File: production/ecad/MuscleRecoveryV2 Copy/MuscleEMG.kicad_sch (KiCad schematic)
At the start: 34 parts, among them J6 Screw_Terminal_01x03, U5 AD8232ACPZ-R7, U7 ADS1115IDGS

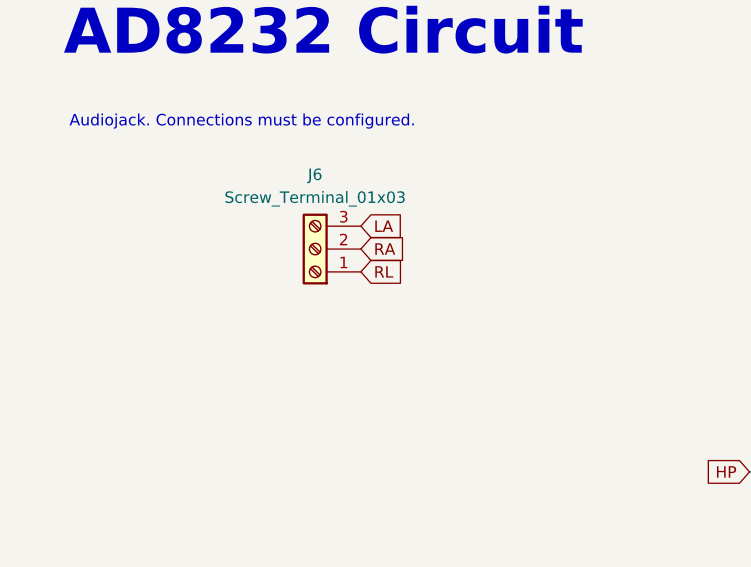
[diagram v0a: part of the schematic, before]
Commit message: Pushing Most of the final changes for PCB REV2
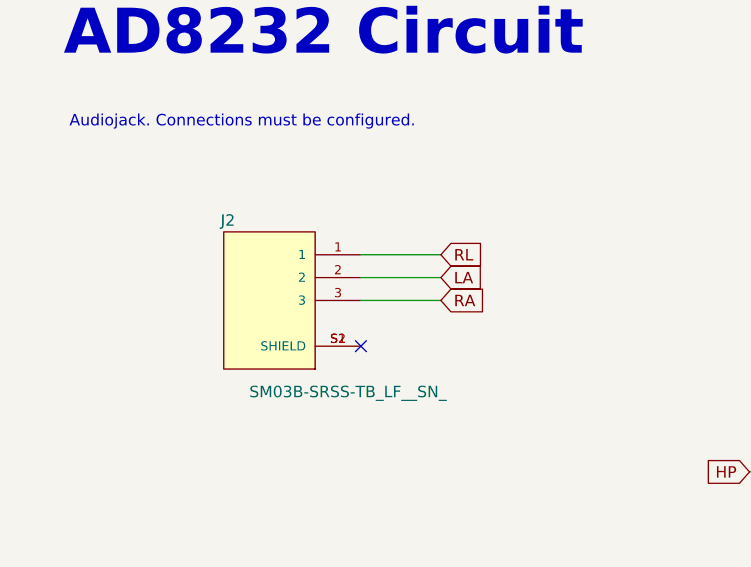
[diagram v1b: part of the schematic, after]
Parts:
- removed J6: Screw_Terminal_01x03, Connector_PinHeader_2.54mm:PinHeader_1x03_P2.54mm_Horizontal, symbol Connector:Screw_Terminal_01x03
- added J2: SM03B-SRSS-TB_LF__SN_, Muscle_Recovery_Footprint_Library:JST_SM03B-SRSS-TB_LF__SN_, symbol MuscleRecoverySymbolLibray:SM03B-SRSS-TB_LF__SN_
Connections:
- net LA: now also J2.2
- net RA: now also J2.3
- net RL: now also J2.1
- new net: J2.S1 (SHIELD), J2.S2 (SHIELD)
- no-connect marks 3 -> 4
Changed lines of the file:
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@@
   (no_connect (at 35.56 172.72))
   (no_connect (at 35.56 170.18))
+  (no_connect (at 52.07 60.96))
   (wire (pts (xy 119.38 52.07) (xy 119.38 49.53))
     (stroke (width 0) (type default))
@@
     (stroke (width 0) (type default))
   )
+  (wire (pts (xy 52.07 55.88) (xy 60.96 55.88))
+    (stroke (width 0) (type default))
+  )
   (wire (pts (xy 219.71 52.07) (xy 245.11 52.07))
     (stroke (width 0) (type default))
@@
     (stroke (width 0) (type default))
   )
+  (wire (pts (xy 52.07 53.34) (xy 60.96 53.34))
+    (stroke (width 0) (type default))
+  )
   (wire (pts (xy 119.38 35.56) (xy 124.46 35.56))
     (stroke (width 0) (type default))
@@
   )
   (wire (pts (xy 125.73 22.86) (xy 128.27 22.86))
+    (stroke (width 0) (type default))
+  )
+  (wire (pts (xy 52.07 50.8) (xy 60.96 50.8))
     (stroke (width 0) (type default))
   )
@@
   (text "ADC" (at 25.4 139.7 0)
     (effects (font (size 5 5) bold) (justify left bottom))
-  )
-  (global_label "RA" (shape input) (at 52.07 50.165 0) (fields_autoplaced)
-    (effects (font (size 1.27 1.27)) (justify left))
-    (property "Intersheetrefs" "${INTERSHEET_REFS}" (at 57.4138 50.165 0)
-      (effects (font (size 1.27 1.27)) (justify left) hide)
-    )
   )
   (global_label "SCL" (shape input) (at 76.2 170.18 0) (fields_autoplaced)
@@
     )
   )
+  (global_label "LA" (shape input) (at 60.96 53.34 0) (fields_autoplaced)
+    (effects (font (size 1.27 1.27)) (justify left))
+    (property "Intersheetrefs" "${INTERSHEET_REFS}" (at 66.0619 53.34 0)
+      (effects (font (size 1.27 1.27)) (justify left) hide)
+    )
+  )
   (global_label "SW" (shape input) (at 144.78 66.04 180) (fields_autoplaced)
     (effects (font (size 1.27 1.27)) (justify right))
@@
     )
   )
-  (global_label "RL" (shape input) (at 52.07 52.705 0) (fields_autoplaced)
-    (effects (font (size 1.27 1.27)) (justify left))
-    (property "Intersheetrefs" "${INTERSHEET_REFS}" (at 57.3533 52.705 0)
-      (effects (font (size 1.27 1.27)) (justify left) hide)
-    )
-  )
   (global_label "ALERT{slash}READY" (shape bidirectional) (at 226.06 156.21 180) (fields_autoplaced)
     (effects (font (size 1.27 1.27)) (justify right))
@@
     )
   )
-  (global_label "LA" (shape input) (at 52.07 47.625 0) (fields_autoplaced)
+  (global_label "RA" (shape input) (at 60.96 55.88 0) (fields_autoplaced)
     (effects (font (size 1.27 1.27)) (justify left))
-    (property "Intersheetrefs" "${INTERSHEET_REFS}" (at 57.1719 47.625 0)
+    (property "Intersheetrefs" "${INTERSHEET_REFS}" (at 66.3038 55.88 0)
       (effects (font (size 1.27 1.27)) (justify left) hide)
     )
@@
     )
   )
+  (global_label "RL" (shape input) (at 60.96 50.8 0) (fields_autoplaced)
+    (effects (font (size 1.27 1.27)) (justify left))
+    (property "Intersheetrefs" "${INTERSHEET_REFS}" (at 66.2433 50.8 0)
+      (effects (font (size 1.27 1.27)) (justify left) hide)
+    )
+  )
   (global_label "LOD+" (shape input) (at 219.71 71.12 0) (fields_autoplaced)
     (effects (font (size 1.27 1.27)) (justify left))
@@
         (path "/4e550305-79d2-4e4a-a502-817ebcc79f9a/284c60dd-e199-4b03-b99f-cc7eaed256f8"
           (reference "C3") (unit 1)
-        )
-      )
-    )
-  )
-  (symbol (lib_id "Connector:Screw_Terminal_01x03") (at 46.99 50.165 180) (unit 1)
-    (in_bom yes) (on_board yes) (dnp no) (fields_autoplaced)
-    (property "Reference" "J6" (at 46.99 41.91 0)
-      (effects (font (size 1.27 1.27)))
-    )
-    (property "Value" "Screw_Terminal_01x03" (at 46.99 44.45 0)
-      (effects (font (size 1.27 1.27)))
-    )
-    (property "Footprint" "Connector_PinHeader_2.54mm:PinHeader_1x03_P2.54mm_Horizontal" (at 46.99 50.165 0)
-      (effects (font (size 1.27 1.27)) hide)
-    )
-    (property "Datasheet" "~" (at 46.99 50.165 0)
-      (effects (font (size 1.27 1.27)) hide)
-    )
-    (pin "1")
-    (pin "2")
-    (pin "3")
-    (instances
-      (project "MuscleRecoveryV1"
-        (path "/4e550305-79d2-4e4a-a502-817ebcc79f9a/284c60dd-e199-4b03-b99f-cc7eaed256f8"
-          (reference "J6") (unit 1)
         )
       )
@@
         )
       )
+    )
+  )
+  (symbol (lib_id "MuscleRecoverySymbolLibray:SM03B-SRSS-TB_LF__SN_") (at 41.91 55.88 0) (mirror y) (unit 1)
+    (in_bom yes) (on_board yes) (dnp no)
+    (property "Reference" "J2" (at 38.1 46.99 0)
+      (effects (font (size 1.27 1.27)) (justify left))
+    )
+    (property "Value" "SM03B-SRSS-TB_LF__SN_" (at 61.595 66.04 0)
+      (effects (font (size 1.27 1.27)) (justify left))
+    )
+    (property "Footprint" "Muscle_Recovery_Footprint_Library:JST_SM03B-SRSS-TB_LF__SN_" (at 34.29 71.12 0)
+      (effects (font (size 1.27 1.27)) (justify bottom) hide)
+    )
+    (property "Datasheet" "" (at 41.91 55.88 0)
+      (effects (font (size 1.27 1.27)) hide)
+    )
+    (property "MF" "JST Sales America Inc." (at 34.29 71.12 0)
+      (effects (font (size 1.27 1.27)) (justify bottom) hide)
+    )
+    (property "Description" "\nConnector Header Surface Mount, Right Angle 3 position 0.039 (1.00mm)\n" (at 34.29 71.12 0)
+      (effects (font (size 1.27 1.27)) (justify bottom) hide)
+    )
+    (property "Package" "None" (at 29.21 62.23 0)
+      (effects (font (size 1.27 1.27)) (justify bottom) hide)
+    )
+    (property "Price" "None" (at 26.67 62.23 0)
+      (effects (font (size 1.27 1.27)) (justify bottom) hide)
+    )
+    (property "Check_prices" "https://www.snapeda.com/parts/SM03B-SRSS-TB(LF)(SN)/JST+Sales+America+Inc./view-part/?ref=eda" (at 34.29 71.12 0)
+      (effects (font (size 1.27 1.27)) (justify bottom) hide)
+    )
+    (property "STANDARD" "Manufacturer Recommendation" (at 34.29 71.12 0)
+      (effects (font (size 1.27 1.27)) (justify bottom) hide)
+    )
+    (property "SnapEDA_Link" "https://www.snapeda.com/parts/SM03B-SRSS-TB(LF)(SN)/JST+Sales+America+Inc./view-part/?ref=snap" (at 34.29 71.12 0)
+      (effects (font (size 1.27 1.27)) (justify bottom) hide)
+    )
+    (property "MP" "SM03B-SRSS-TB(LF)(SN)" (at 34.29 71.12 0)
+      (effects (font (size 1.27 1.27)) (justify bottom) hide)
+    )
+    (property "Availability" "In Stock" (at 29.21 58.42 0)
+      (effects (font (size 1.27 1.27)) (justify bottom) hide)
+    )
+    (property "MANUFACTURER" "JST" (at 27.94 60.96 0)
+      (effects (font (size 1.27 1.27)) (justify bottom) hide)
+    )
+    (pin "1")
+    (pin "2")
+    (pin "3")
+    (pin "S1")
+    (pin "S2")
+    (instances
+      (project "MuscleRecoveryV1"
+        (path "/4e550305-79d2-4e4a-a502-817ebcc79f9a/284c60dd-e199-4b03-b99f-cc7eaed256f8"
+          (reference "J2") (unit 1)
+        )
+      )

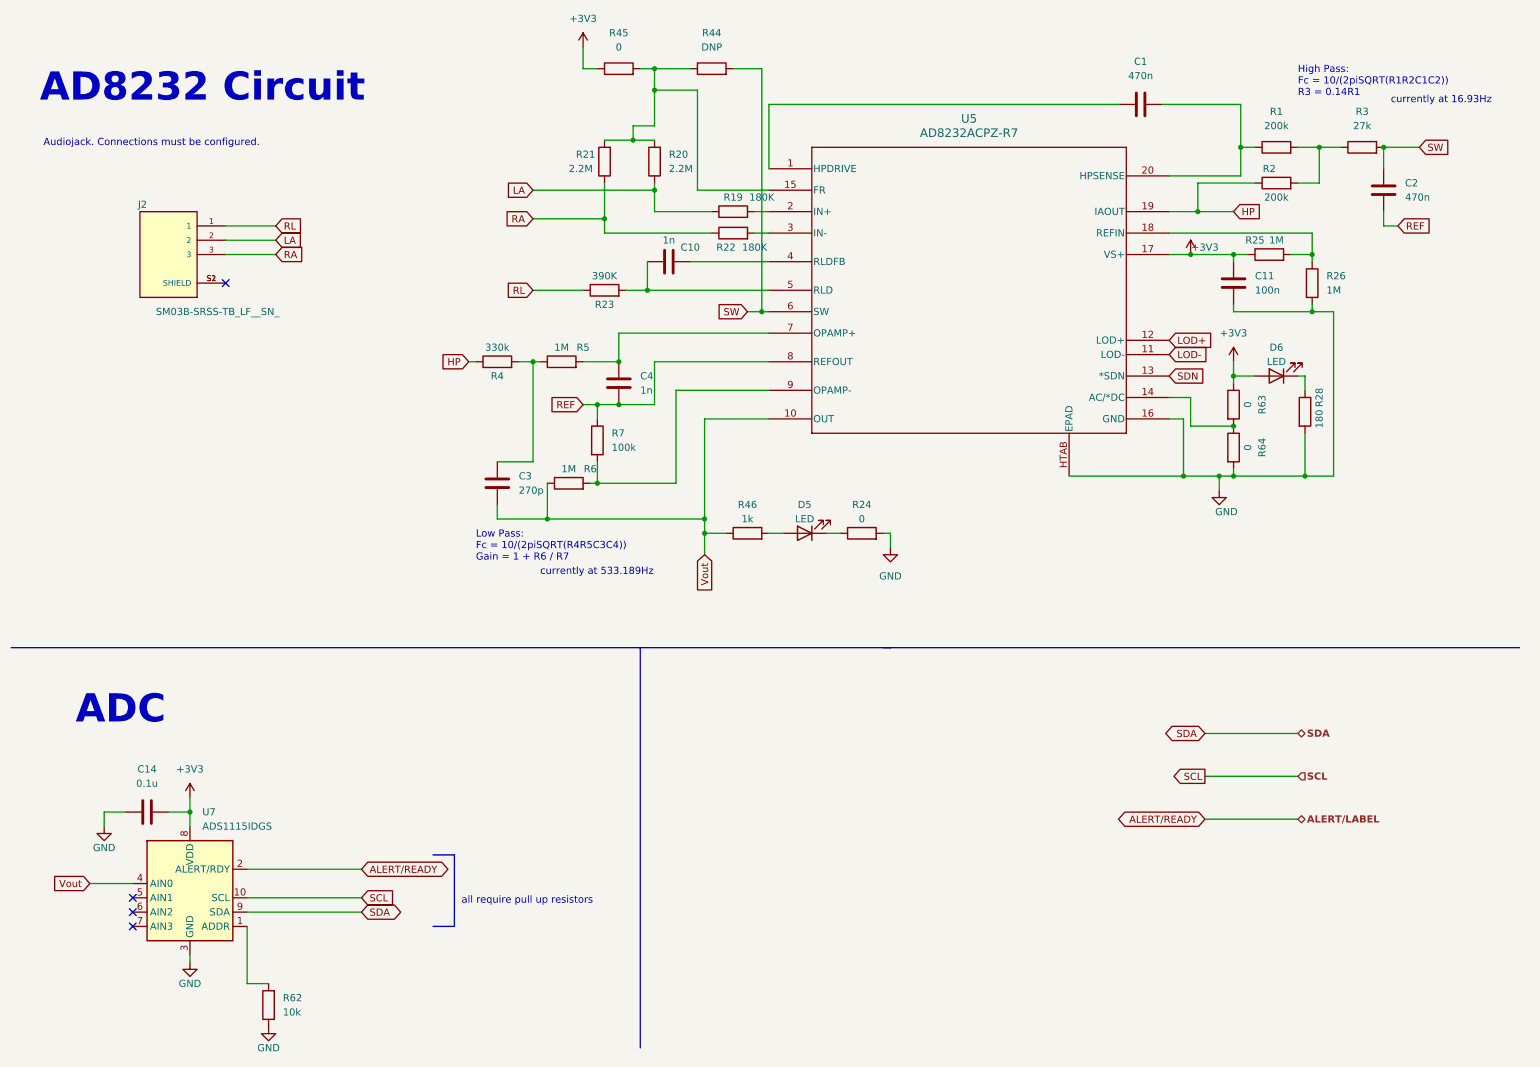
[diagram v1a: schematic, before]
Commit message: Pushing changes post schematic review
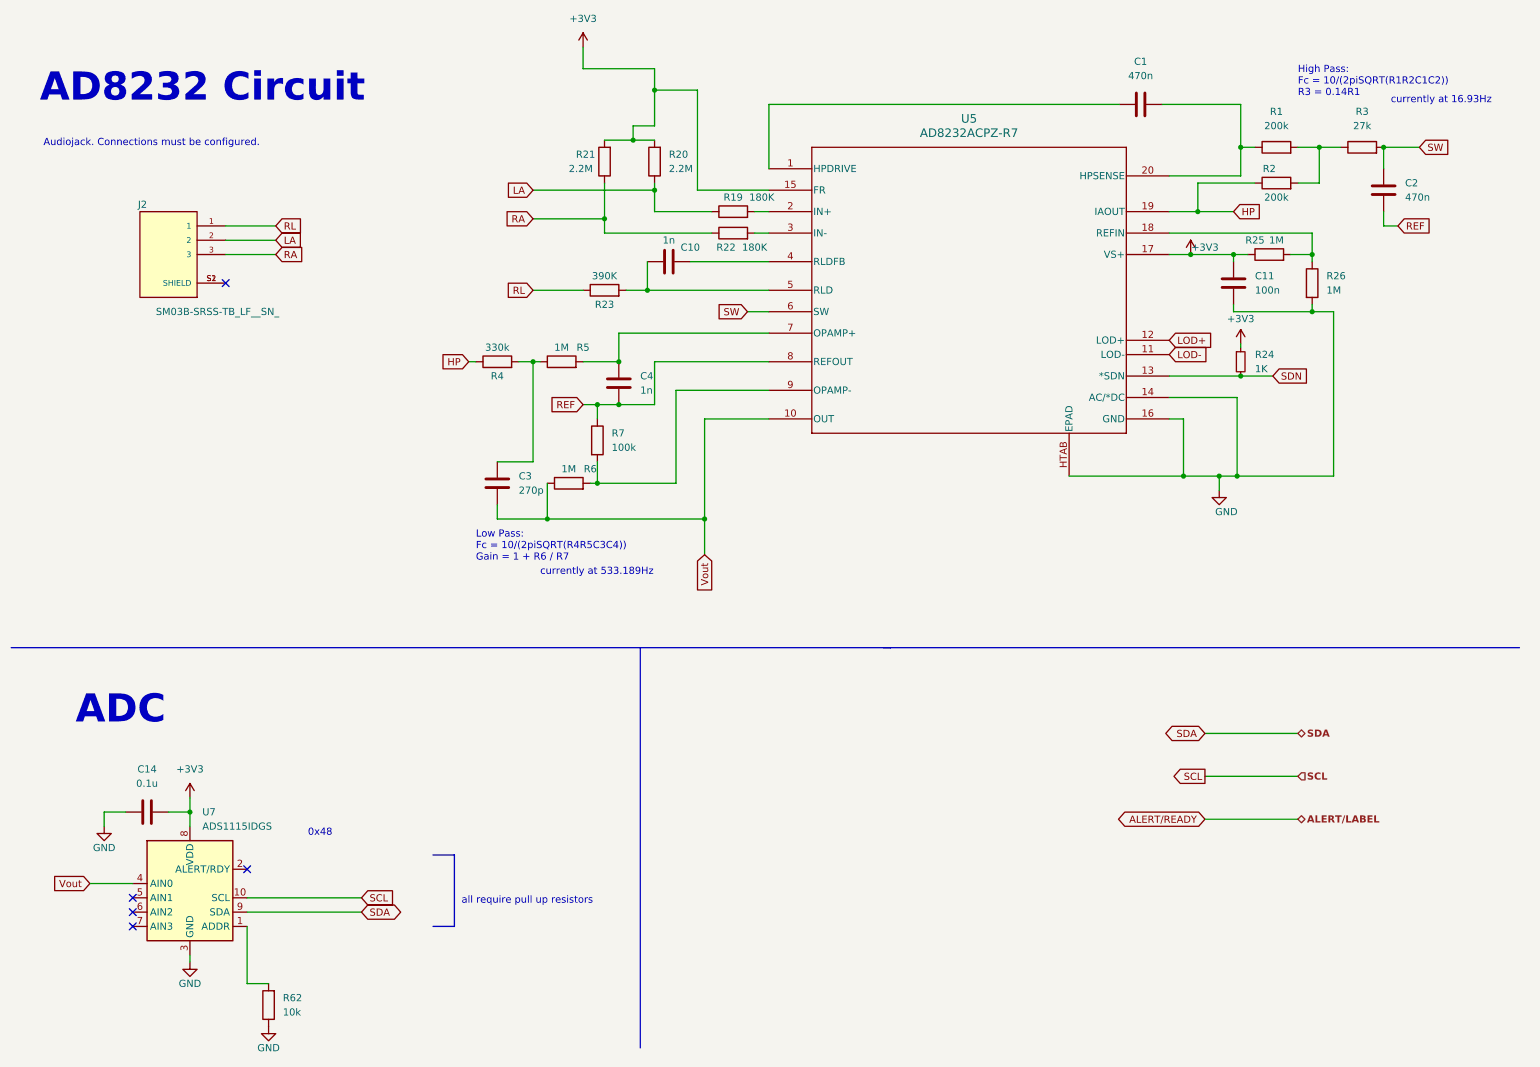
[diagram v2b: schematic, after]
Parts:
- removed D5, D6: LED, LED_SMD:LED_0402_1005Metric, symbol Device:LED
- removed R24, R45, R63, R64: 0, Resistor_SMD:R_0402_1005Metric, symbol Device:R
- removed R28: 180, Resistor_SMD:R_0402_1005Metric, symbol Device:R
- removed R44: DNP, Resistor_SMD:R_0402_1005Metric, symbol Device:R
- removed R46: 1k, Resistor_SMD:R_0402_1005Metric, symbol Device:R
- added R24: 1K, symbol Device:R_Small
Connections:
- net +3V3: now also R20.2, R21.2, U5.15 (FR), R24.1
- net ALERT/READY: no longer U7.2 (ALERT/RDY)
- net GND: now also U5.14 (AC/*DC)
- net SDN: now also R24.2
- no-connect marks 4 -> 5
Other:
- note added: "0x48"
